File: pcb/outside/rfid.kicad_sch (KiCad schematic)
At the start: 25 parts, among them U2 MFRC52201HN1,157, Y1 27.12MHz

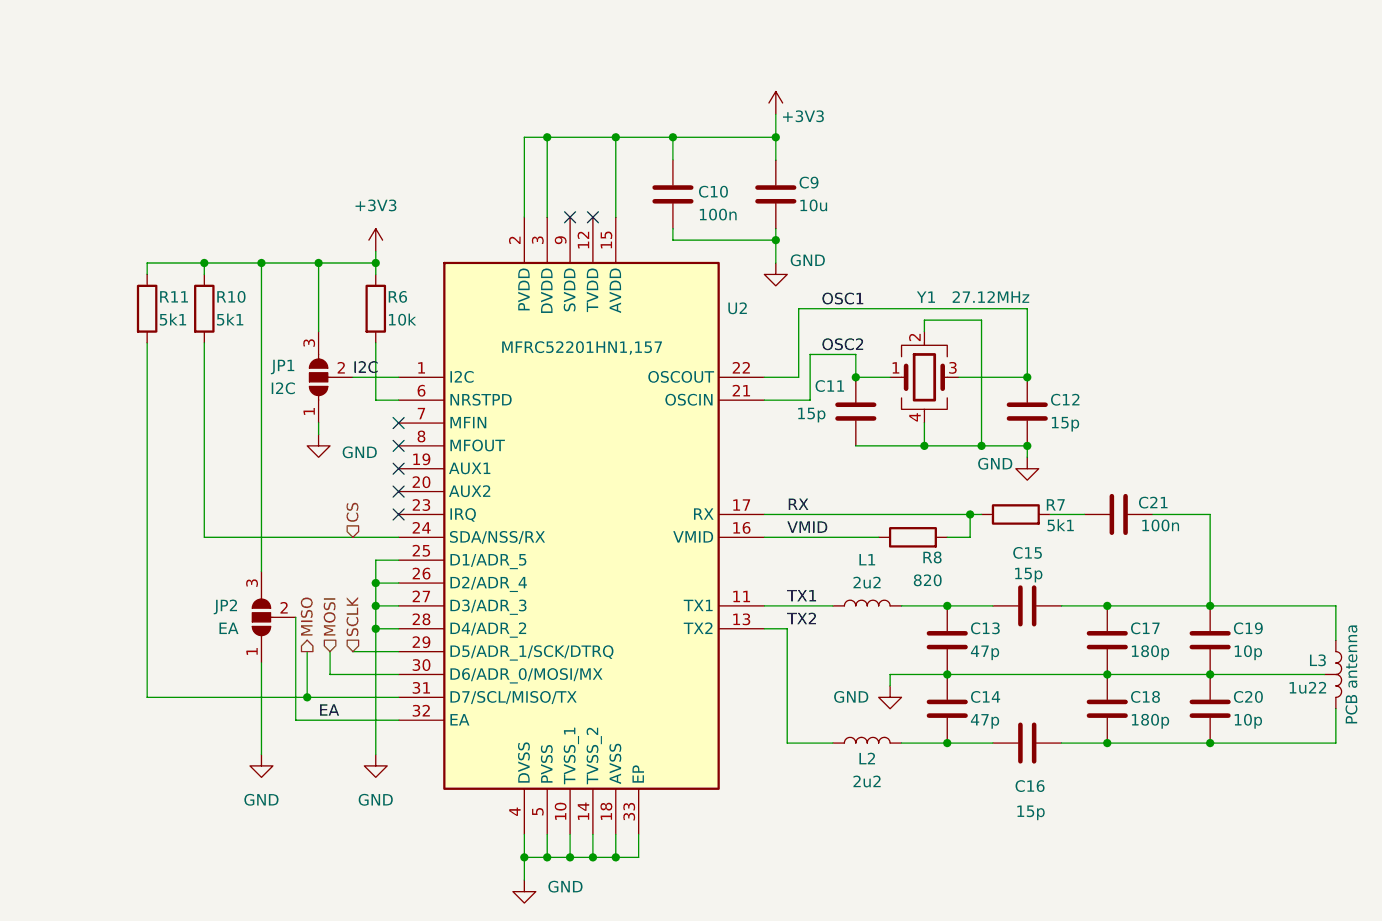
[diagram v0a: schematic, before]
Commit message: feat: add testpoints and rearrange schematic
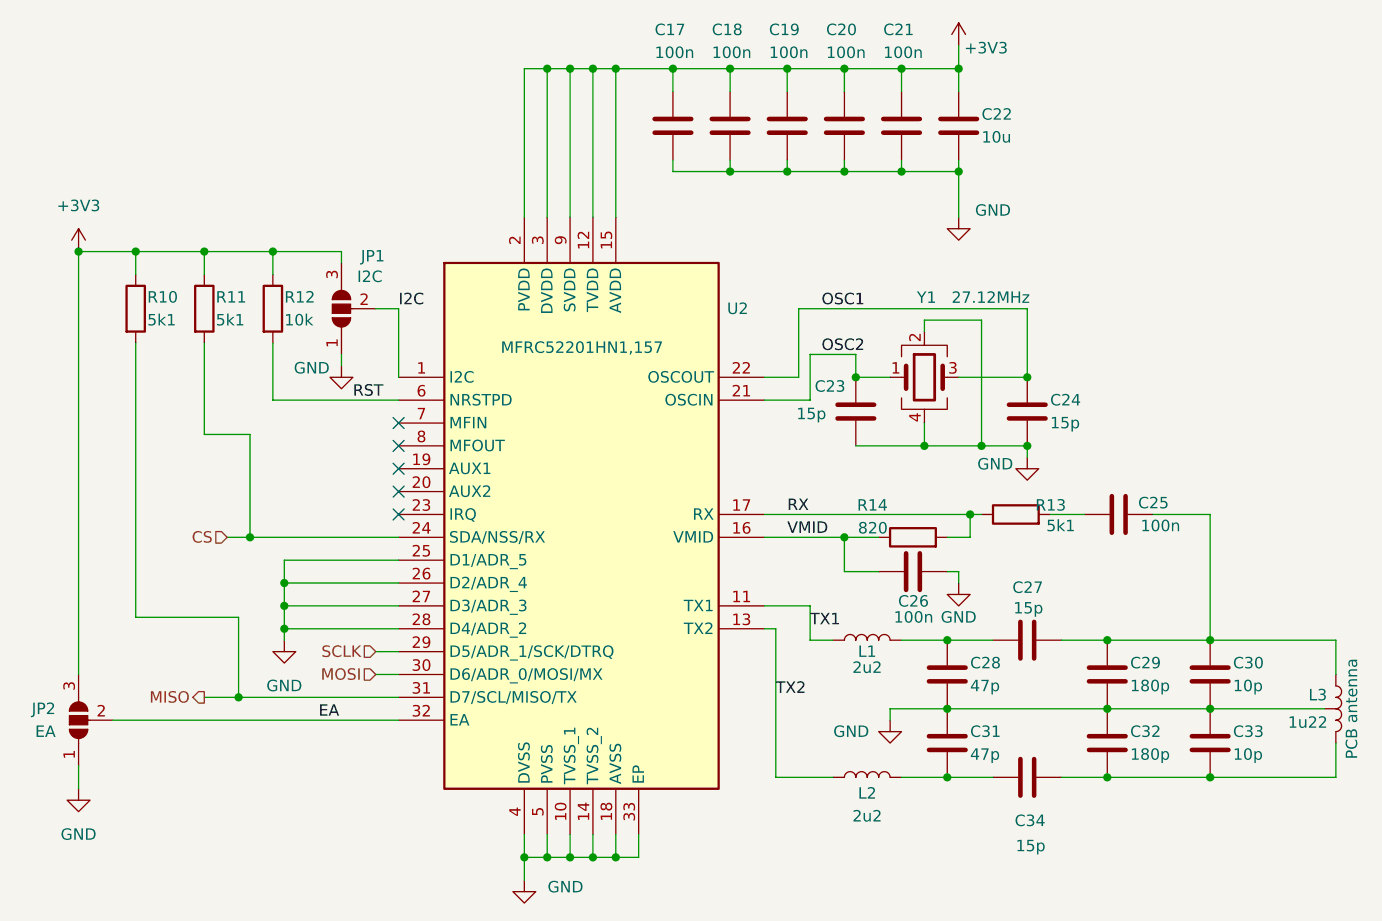
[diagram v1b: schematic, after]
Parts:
- added C18, C19, C20, C21, C26: 100n, Capacitor_SMD:C_0603_1608Metric, symbol Device:C
- renumbered C10 to C17, C9 to C22, C11 to C23, C12 to C24, C21 to C25, C15 to C27, C13 to C28, C17 to C29, C19 to C30, C14 to C31, C18 to C32, C20 to C33, C16 to C34, R11 to R10, R10 to R11, R6 to R12, R7 to R13, R8 to R14
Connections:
- net +3V3: now also U2.12 (TVDD), U2.9 (SVDD), C18.1, C19.1, C20.1, C21.1
- net GND: now also C18.2, C19.2, C20.2, C21.2, C26.2
- net VMID: now also C26.1
- net RST: now reaches R12.2, U2.6 (NRSTPD)
- no-connect marks 7 -> 5
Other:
- moved on the sheet: C17, C22, C27, C28, C29, C30, C31, C32, C33, C34, JP1, JP2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
